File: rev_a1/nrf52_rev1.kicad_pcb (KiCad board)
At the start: 2 copper layers, 48.3 x 48.3 mm, 31 parts, among them P1 CONN_01X18, P2 CONN_01X18, P3 USB_OTG, U1 nRF52832, U2 CP2102, U3 LT1129CST-3.3, Y1 32K, Y2 32M

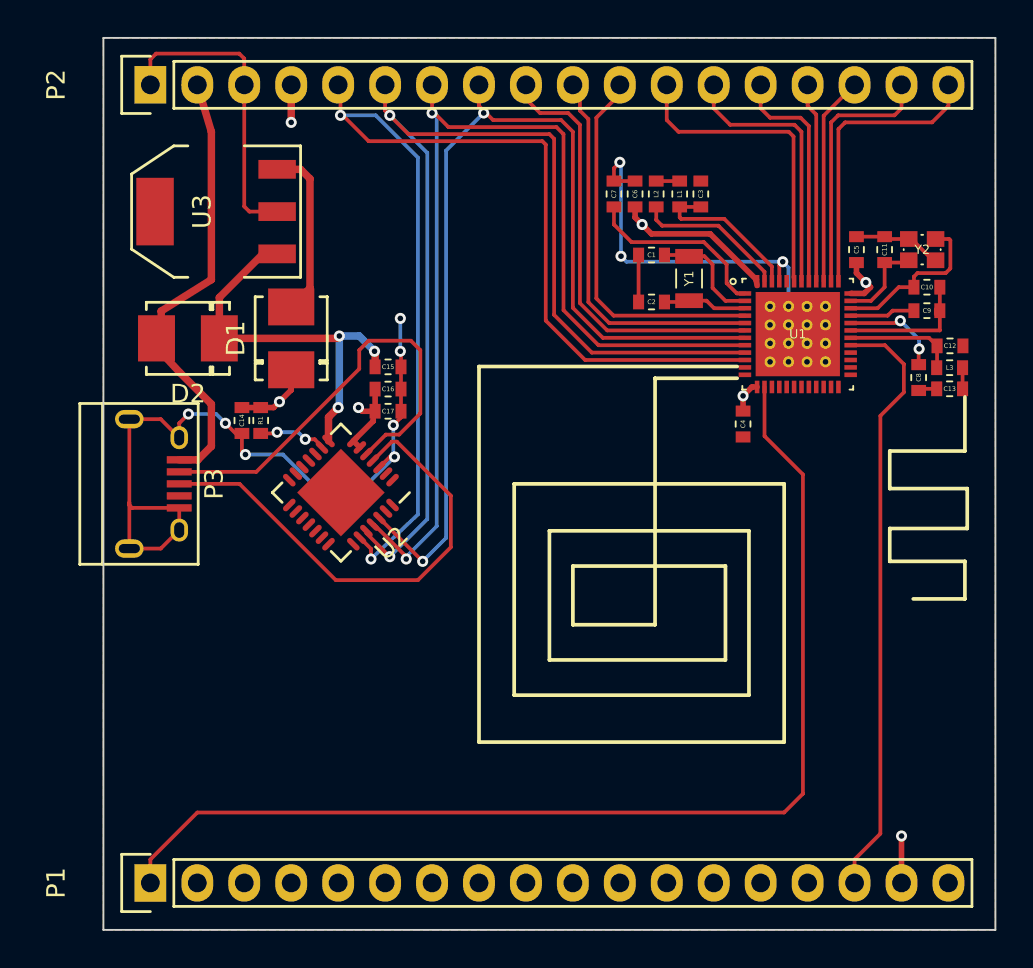
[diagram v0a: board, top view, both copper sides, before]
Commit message: Made the design great again
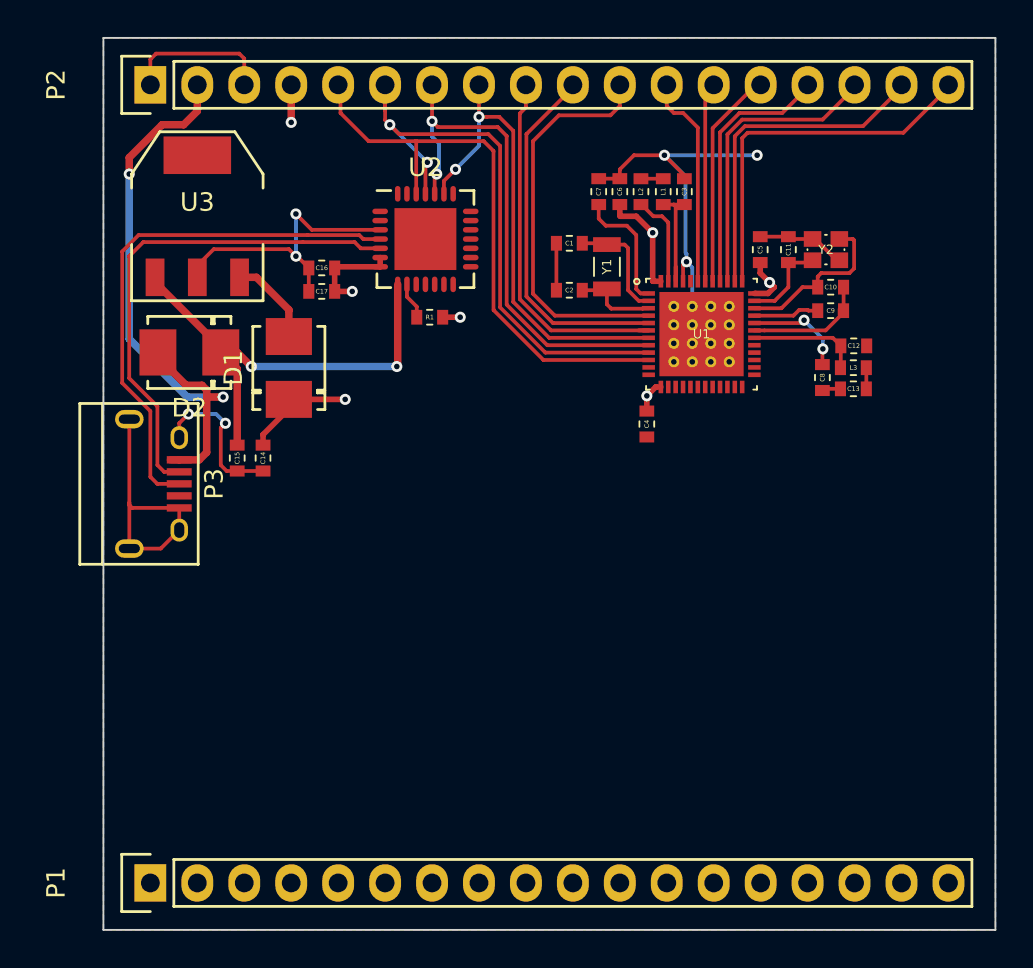
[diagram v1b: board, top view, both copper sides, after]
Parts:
- moved U2 14.5 mm to (42.8, 36.3), turned to 0 degrees
- moved R1 10.7 mm to (43.1, 40.5), turned to 0 degrees
- moved C15 9.54 mm to (32.6, 48.1), turned to 90 degrees
- moved C16 7.47 mm to (37.2, 37.8), turned to 0 degrees
- moved C17 7.41 mm to (37.2, 39.1), turned to 0 degrees
- moved C11 5.21 mm to (62.5, 36.9)
- moved C4 5.21 mm to (54.8, 46.3)
- moved C5 5.21 mm to (60.9, 36.9)
- moved U1 5.21 mm to (57.8, 41.4)
- moved C10 5.21 mm to (64.7, 38.9)
- moved C12 5.21 mm to (66.0, 42.1)
- moved C13 5.21 mm to (66.0, 44.4)
- moved C8 5.21 mm to (64.3, 43.8)
- moved C9 5.21 mm to (64.7, 40.2)
- moved L3 5.21 mm to (66.0, 43.2)
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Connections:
- U2 pad 23: P0.08 -> P0.05
- U2 pad 24: P0.07 -> P0.06
- U2 pad 25: P0.06 -> P0.07
- U2 pad 26: P0.05 -> P0.08
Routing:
- net P0.11: track 60.9 -> 0.00 mm
- net P0.24: track 32.5 -> 0.00 mm
- net P0.08: track 64.8 -> 32.5 mm, vias 2 -> 0
- net P0.05: track 55.4 -> 26.2 mm
- net P0.06: track 56.9 -> 28.3 mm
- net P0.07: track 59.3 -> 32.5 mm
- net GND: track 120.1 -> 109.0 mm, vias 10 -> 7
- net 5V_IN: track 25.0 -> 33.0 mm, vias 0 -> 2
- net P0.31: track 17.0 -> 11.6 mm
- net P0.27: track 11.3 -> 16.0 mm
- net Net-(D1-Pad2): track 9.35 -> 4.84 mm
- net P0.25: track 15.8 -> 20.2 mm
- net P0.26: track 14.0 -> 18.1 mm
- net +5V: track 22.5 -> 26.3 mm, vias 3 -> 2
- net P0.30: track 14.6 -> 10.8 mm
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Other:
- net class Default: clearance 0.0762 -> 0.1524
- rule trace_clearance: 0.0762 -> 0.1524
